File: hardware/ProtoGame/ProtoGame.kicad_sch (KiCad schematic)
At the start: 36 parts, among them J1 SD_Card_Module, SW1 SW_DPST_x2, SW10 SW_MEC_5E, SW2 SW_MEC_5E, SW3 SW_MEC_5E, SW4 SW_MEC_5E, SW5 SW_MEC_5E, SW6 SW_MEC_5E, SW7 SW_MEC_5E, SW8 SW_MEC_5E, SW9 SW_MEC_5E, U1 STM32F103C8Tx - MODULE, U2 AMS1117-3.3

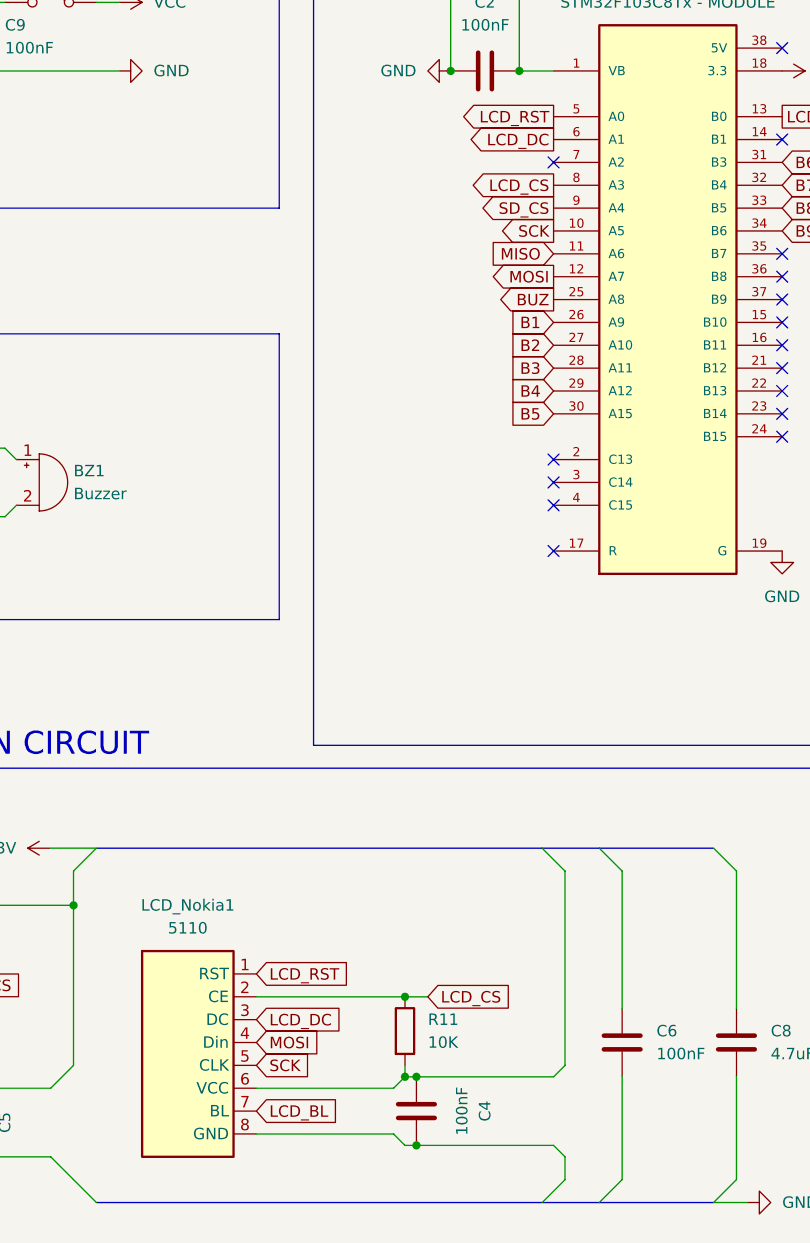
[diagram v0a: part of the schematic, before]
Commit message: little bit refactor in schematic
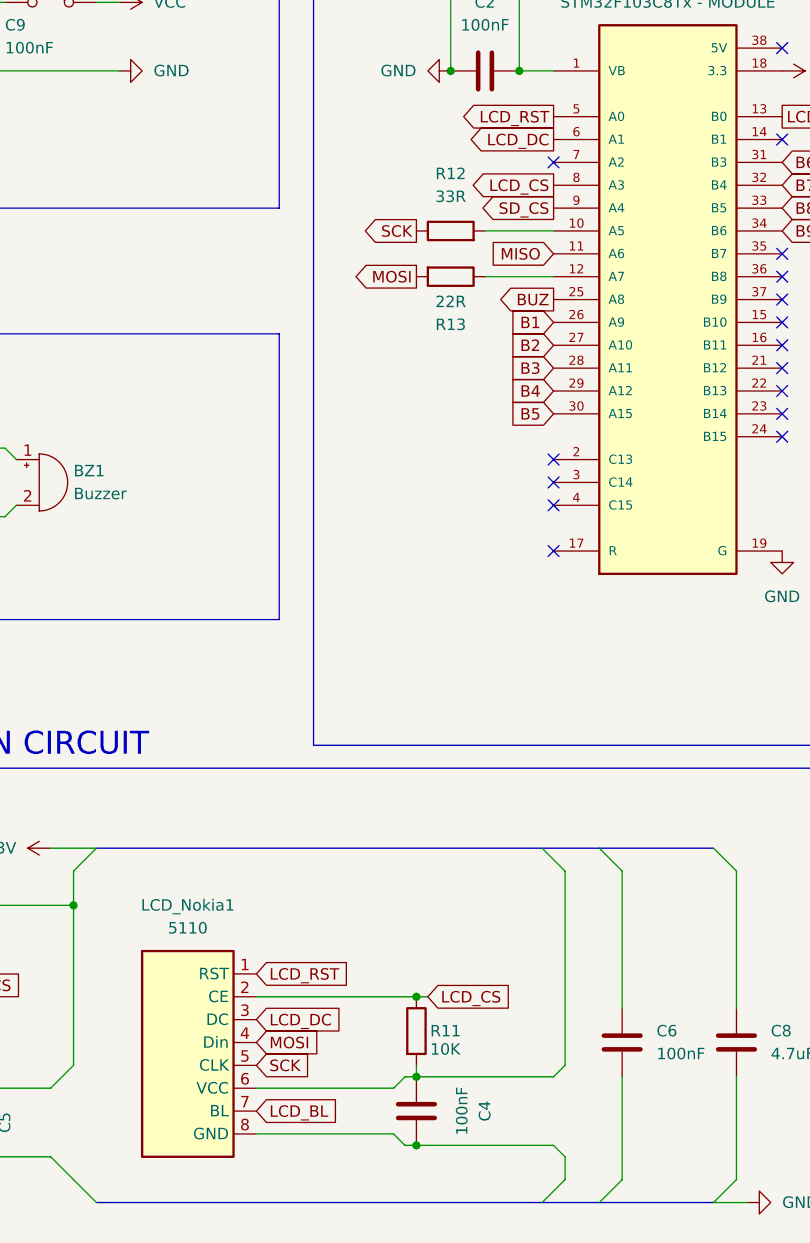
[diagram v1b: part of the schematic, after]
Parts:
- added R12: 33R, Resistor_THT:R_Axial_DIN0207_L6.3mm_D2.5mm_P7.62mm_Horizontal, symbol Device:R
- added R13: 22R, Resistor_THT:R_Axial_DIN0207_L6.3mm_D2.5mm_P7.62mm_Horizontal, symbol Device:R
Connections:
- net MOSI: now also R13.2; no longer U1.12 (A7)
- net SCK: now also R12.1; no longer U1.10 (A5)
- new net: R13.1, U1.12 (A7)
- new net: R12.2, U1.10 (A5)
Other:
- moved on the sheet: R11
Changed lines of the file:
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@@
 	)
 	(junction
-		(at 116.84 163.83)
-		(diameter 0)
-		(color 0 0 0 0)
-	)
-	(junction
 		(at 257.81 110.49)
 		(diameter 0)
@@
 	)
 	(junction
-		(at 55.88 60.96)
+		(at 118.11 163.83)
 		(diameter 0)
 		(color 0 0 0 0)
 	)
 	(junction
-		(at 118.11 180.34)
+		(at 55.88 60.96)
 		(diameter 0)
 		(color 0 0 0 0)
 	)
 	(junction
-		(at 234.95 110.49)
+		(at 118.11 180.34)
 		(diameter 0)
 		(color 0 0 0 0)
 	)
 	(junction
-		(at 116.84 172.72)
+		(at 234.95 110.49)
 		(diameter 0)
 		(color 0 0 0 0)
@@
 	(wire
 		(pts
-			(xy 118.11 172.72) (xy 116.84 172.72)
+			(xy 234.95 140.97) (xy 234.95 142.24)
 		)
 		(stroke
@@
 	(wire
 		(pts
-			(xy 234.95 140.97) (xy 234.95 142.24)
+			(xy 60.96 179.07) (xy 59.69 179.07)
 		)
 		(stroke
@@
 	(wire
 		(pts
-			(xy 60.96 179.07) (xy 59.69 179.07)
+			(xy 125.73 78.74) (xy 133.35 78.74)
 		)
 		(stroke
@@
 	(wire
 		(pts
+			(xy 125.73 83.82) (xy 133.35 83.82)
+		)
+		(stroke
+			(width 0)
+			(type default)
+		)
+	)
+	(wire
+		(pts
 			(xy 220.98 99.06) (xy 220.98 87.63)
 		)
@@
 	(wire
 		(pts
-			(xy 116.84 163.83) (xy 119.38 163.83)
-		)
-		(stroke
-			(width 0)
-			(type default)
-		)
-	)
-	(wire
-		(pts
 			(xy 129.54 48.26) (xy 129.54 60.96)
 		)
@@
 	(wire
 		(pts
-			(xy 116.84 163.83) (xy 100.33 163.83)
+			(xy 100.33 163.83) (xy 118.11 163.83)
 		)
 		(stroke
@@
 	(wire
 		(pts
-			(xy 116.84 171.45) (xy 116.84 172.72)
+			(xy 118.11 171.45) (xy 118.11 172.72)
 		)
 		(stroke
@@
 	(wire
 		(pts
+			(xy 118.11 172.72) (xy 116.84 172.72)
+		)
+		(stroke
+			(width 0)
+			(type default)
+		)
+	)
+	(wire
+		(pts
 			(xy 198.12 130.81) (xy 201.93 130.81)
 		)
@@
 	(wire
 		(pts
+			(xy 118.11 163.83) (xy 119.38 163.83)
+		)
+		(stroke
+			(width 0)
+			(type default)
+		)
+	)
+	(wire
+		(pts
 			(xy 118.11 172.72) (xy 133.35 172.72)
 		)
@@
 	(global_label "SCK"
 		(shape output)
-		(at 133.35 78.74 180)
+		(at 118.11 78.74 180)
 		(fields_autoplaced yes)
 		(effects
@@
 		)
 		(property "Intersheetrefs" "${INTERSHEET_REFS}"
-			(at 126.6153 78.74 0)
+			(at 111.3753 78.74 0)
 			(effects
 				(font
@@
 	(global_label "MOSI"
 		(shape output)
-		(at 133.35 83.82 180)
+		(at 118.11 83.82 180)
 		(fields_autoplaced yes)
 		(effects
@@
 		)
 		(property "Intersheetrefs" "${INTERSHEET_REFS}"
-			(at 125.7686 83.82 0)
+			(at 110.5286 83.82 0)
 			(effects
 				(font
@@
 	(symbol
 		(lib_id "Device:R")
+		(at 121.92 83.82 270)
+		(unit 1)
+		(exclude_from_sim no)
+		(in_bom yes)
+		(on_board yes)
+		(dnp no)
+		(property "Reference" "R13"
+			(at 121.92 89.154 90)
+			(effects
+				(font
+					(size 1.27 1.27)
+				)
+			)
+		)
+		(property "Value" "22R"
+			(at 121.92 86.614 90)
+			(effects
+				(font
+					(size 1.27 1.27)
+				)
+			)
+		)
+		(property "Footprint" "Resistor_THT:R_Axial_DIN0207_L6.3mm_D2.5mm_P7.62mm_Horizontal"
+			(at 121.92 82.042 90)
+			(effects
+				(font
+					(size 1.27 1.27)
+				)
+				(hide yes)
+			)
+		)
+		(property "Datasheet" "~"
+			(at 121.92 83.82 0)
+			(effects
+				(font
+					(size 1.27 1.27)
+				)
+				(hide yes)
+			)
+		)
+		(property "Description" "Resistor"
+			(at 121.92 83.82 0)
+			(effects
+				(font
+					(size 1.27 1.27)
+				)
+				(hide yes)
+			)
+		)
+		(pin "1"
+		)
+		(pin "2"
+		)
+		(instances
+			(project "ProtoGame"
+				(path "/2f633d8f-de1b-4944-902d-f651e9a8378a"
+					(reference "R13")
+					(unit 1)
+				)
+			)
+		)
+	)
+	(symbol
+		(lib_id "Device:R")
 		(at 257.81 73.66 0)
 		(unit 1)
@@
 	)
 	(symbol
+		(lib_id "Device:R")
+		(at 121.92 78.74 90)
+		(unit 1)
+		(exclude_from_sim no)
+		(in_bom yes)
+		(on_board yes)
+		(dnp no)
+		(fields_autoplaced yes)
+		(property "Reference" "R12"
+			(at 121.92 72.39 90)
+			(effects
+				(font
+					(size 1.27 1.27)
+				)
+			)
+		)
+		(property "Value" "33R"
+			(at 121.92 74.93 90)
+			(effects
+				(font
+					(size 1.27 1.27)
+				)
+			)
+		)
+		(property "Footprint" "Resistor_THT:R_Axial_DIN0207_L6.3mm_D2.5mm_P7.62mm_Horizontal"
+			(at 121.92 80.518 90)
+			(effects
+				(font
+					(size 1.27 1.27)
+				)
+				(hide yes)
+			)
+		)
+		(property "Datasheet" "~"
+			(at 121.92 78.74 0)
+			(effects
+				(font
+					(size 1.27 1.27)
+				)
+				(hide yes)
+			)
+		)
+		(property "Description" "Resistor"
+			(at 121.92 78.74 0)
+			(effects
+				(font
+					(size 1.27 1.27)
+				)
+				(hide yes)
+			)
+		)
+		(pin "1"
+		)
+		(pin "2"
+		)
+		(instances
+			(project ""
+				(path "/2f633d8f-de1b-4944-902d-f651e9a8378a"
+					(reference "R12")
+					(unit 1)
+				)
+			)
+		)
+	)
+	(symbol
 		(lib_id "Switch:SW_MEC_5E")
 		(at 229.87 101.6 0)
@@
 	(symbol
 		(lib_id "Device:R")
-		(at 116.84 167.64 0)
+		(at 118.11 167.64 0)
 		(unit 1)
 		(exclude_from_sim no)
@@
 		(on_board yes)
 		(dnp no)
-		(fields_autoplaced yes)
 		(property "Reference" "R11"
-			(at 119.38 166.3699 0)
+			(at 119.634 167.64 0)
 			(effects
 				(font
@@
 		)
 		(property "Value" "10K"
-			(at 119.38 168.9099 0)
+			(at 119.634 169.672 0)
 			(effects
 				(font
@@
 		)
 		(property "Footprint" "Resistor_THT:R_Axial_DIN0207_L6.3mm_D2.5mm_P7.62mm_Horizontal"
-			(at 115.062 167.64 90)
+			(at 116.332 167.64 90)
 			(effects
 				(font
@@
 		)
 		(property "Datasheet" "~"
-			(at 116.84 167.64 0)
+			(at 118.11 167.64 0)
 			(effects
 				(font
@@
 		)
 		(property "Description" "Resistor"
-			(at 116.84 167.64 0)
+			(at 118.11 167.64 0)
 			(effects
 				(font
